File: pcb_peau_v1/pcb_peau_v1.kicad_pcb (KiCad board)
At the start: 2 copper layers, 76 x 74 mm, 27 parts, among them J1 Conn_01x05, J2 Conn_01x05, J4 Conn_02x08_Top_Bottom, J5 Conn_02x12_Top_Bottom, U1 REF200AU, U2 TLC274, U3 CD74HC4067SM, U4 CD74HC4067SM, U5 CD74HC4067SM, U6 CD74HC4067SM, U7 TLC274, U8 TLC274, U9 TLC274

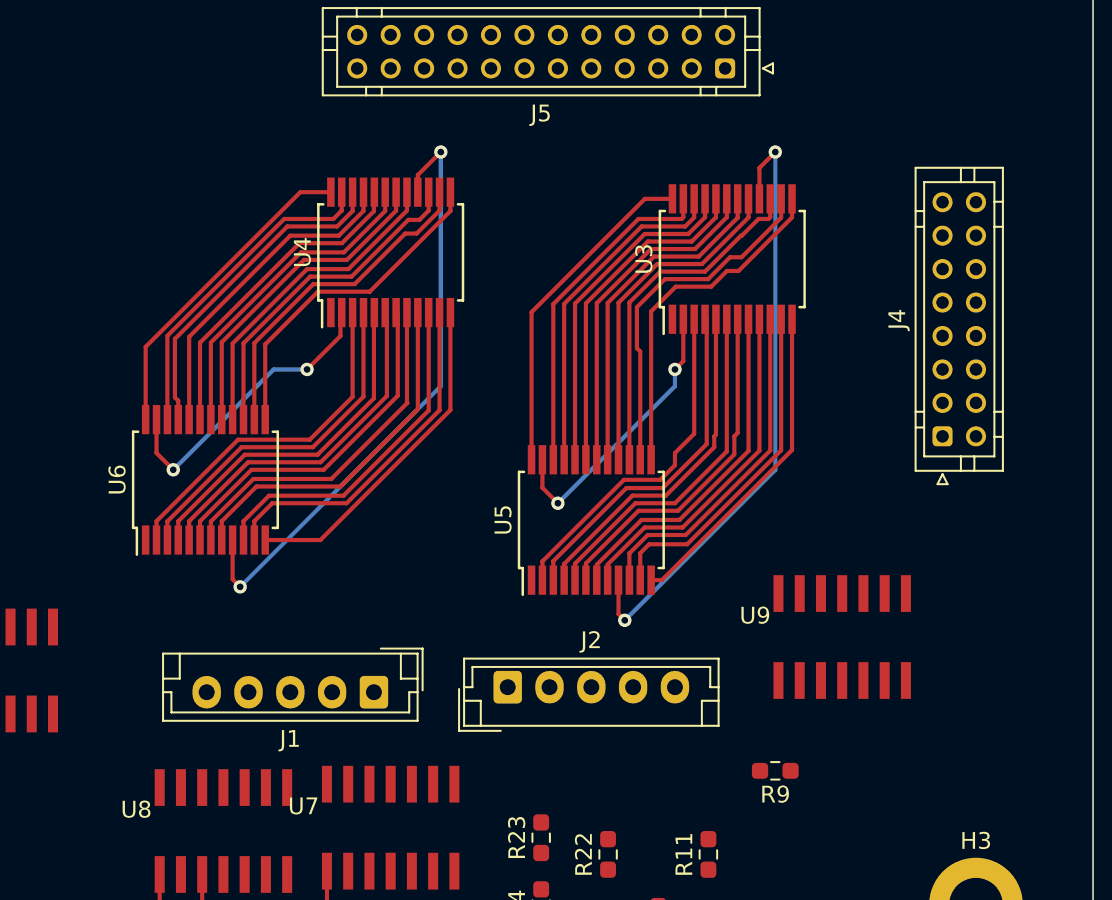
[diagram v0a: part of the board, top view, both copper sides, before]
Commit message: PCB avancé
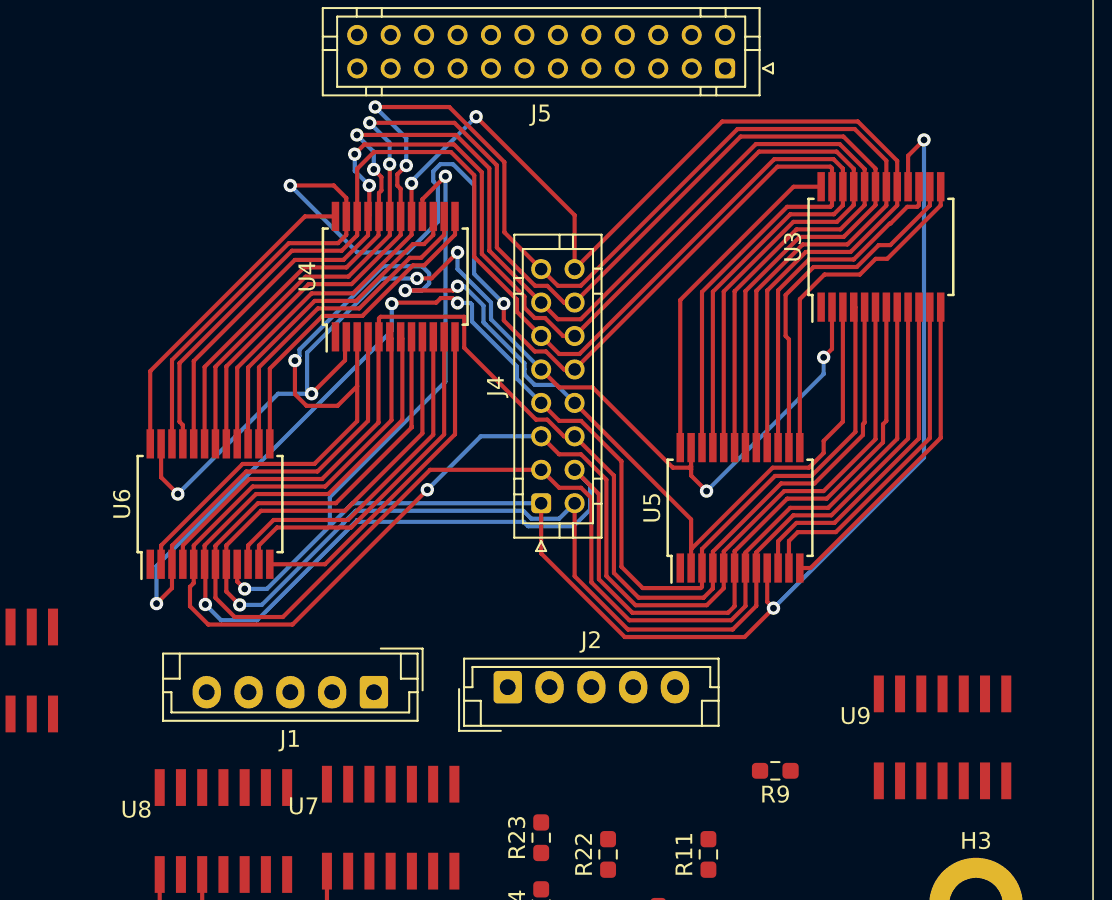
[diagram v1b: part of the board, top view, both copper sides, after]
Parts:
- moved J4 24.3 mm to (210.0, 86.0)
- moved U5 8.92 mm to (221.9, 86.3)
- moved U3 8.92 mm to (230.3, 70.7)
- moved U9 8.49 mm to (234.0, 100.0)
- moved U4 1.48 mm to (201.3, 72.5)
- moved U6 1.48 mm to (190.2, 86.0)
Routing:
- net Net-(J4-Pin_7): track 41.7 -> 100.1 mm, vias 0 -> 3
- net Net-(J4-Pin_10): track 40.0 -> 98.1 mm, vias 0 -> 2
- net Net-(J4-Pin_15): track 39.8 -> 91.1 mm, vias 0 -> 2
- net Net-(J4-Pin_4): track 41.8 -> 92.0 mm, vias 0 -> 1
- net Net-(J4-Pin_14): track 39.8 -> 89.4 mm, vias 0 -> 2
- net Net-(J4-Pin_13): track 39.8 -> 89.1 mm, vias 0 -> 2
- net Net-(J4-Pin_5): track 41.8 -> 90.6 mm, vias 0 -> 1
- net Net-(J4-Pin_12): track 40.0 -> 88.2 mm, vias 0 -> 2
- net Net-(J4-Pin_3): track 41.9 -> 89.0 mm
- net Net-(J4-Pin_11): track 40.2 -> 86.9 mm
- net Net-(J4-Pin_8): track 41.6 -> 86.8 mm, vias 0 -> 3
- net Net-(J4-Pin_2): track 42.1 -> 87.2 mm, vias 0 -> 1
- net Net-(J4-Pin_16): track 39.8 -> 84.3 mm, vias 0 -> 2
- net Net-(J4-Pin_9): track 35.2 -> 70.0 mm, vias 4 -> 6
- net Net-(J4-Pin_6): track 41.5 -> 75.6 mm
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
